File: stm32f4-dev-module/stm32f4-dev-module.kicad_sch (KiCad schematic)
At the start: 38 parts, among them J1 SW, J2 Screw_Terminal_CAN, J3 I2C1, J4 SPI1, P1 USB_C_Plug, SW1 SW_SPST, SW2 SW_SPDT, U1 STM32F405RGT6, U2 USBLC6-2SC6, U3 SN65HVD230, U4 AP2112K-3.3, U5 ICM-42670-P, Y1 25MHz

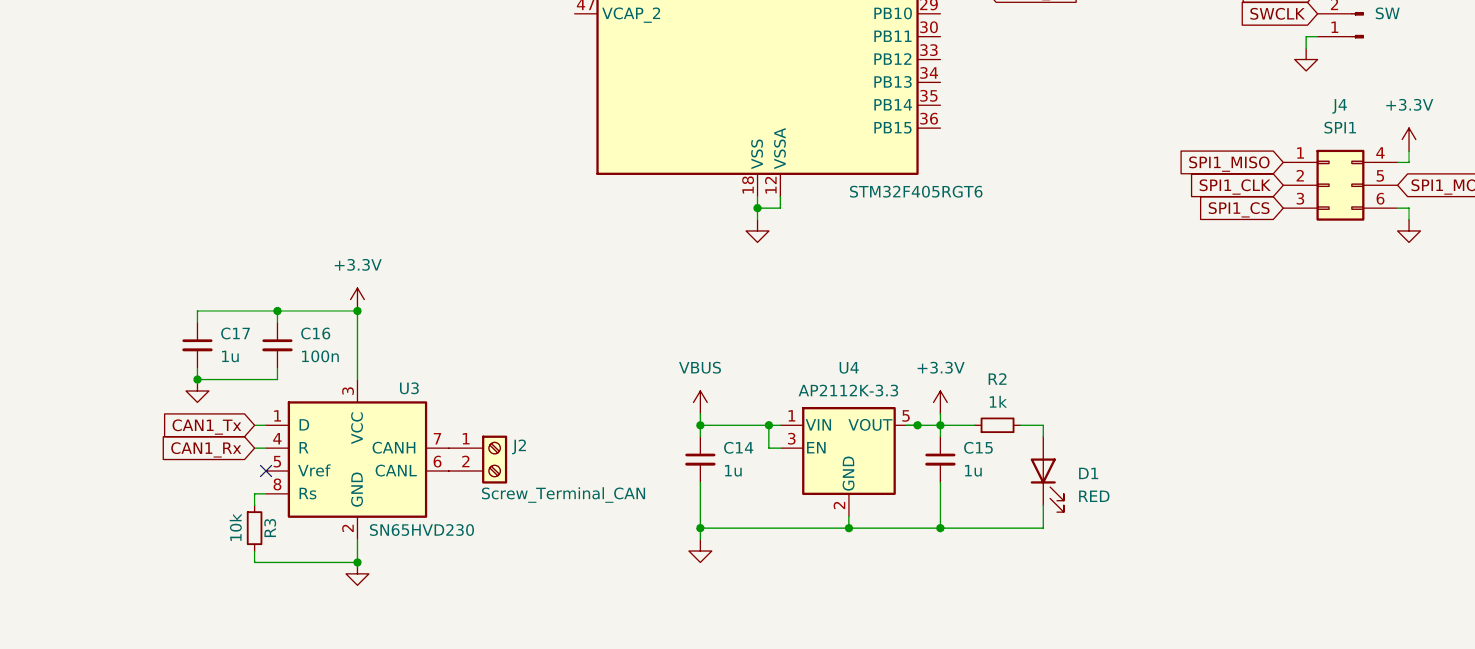
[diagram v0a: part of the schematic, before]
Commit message: commit
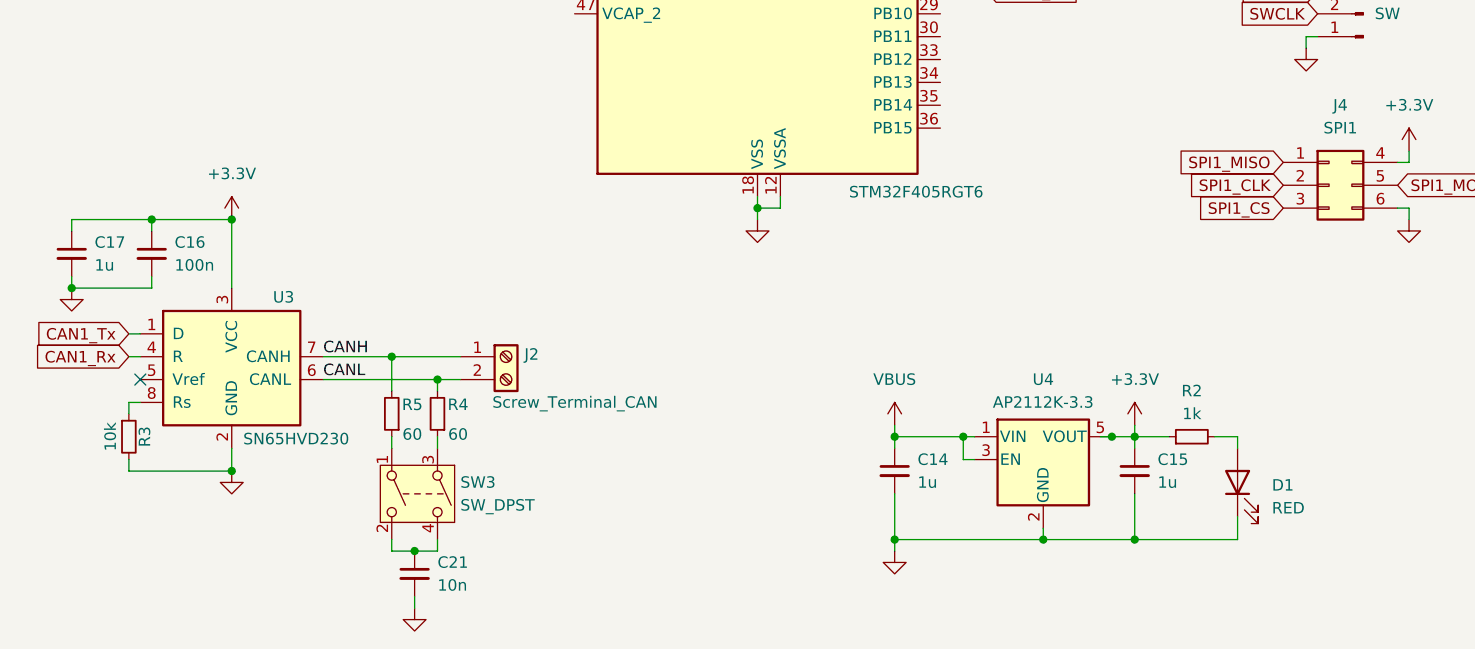
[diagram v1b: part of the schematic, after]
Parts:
- added C21: 10n, symbol Device:C_Small
- added R4, R5: 60, symbol Device:R_Small
- added SW3: SW_DPST, symbol Switch:SW_DPST
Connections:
- net GND: now also C21.2
- net CANH: now reaches J2.1 (Pin_1), U3.7 (CANH)
- net CANH: now also R5.2
- net CANL: now reaches J2.2 (Pin_2), U3.6 (CANL)
- net CANL: now also R4.2
- new net: R5.1, SW3.1
- new net: C21.1, SW3.2, SW3.4
- new net: R4.1, SW3.3
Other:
- moved on the sheet: C14, C15, C16, C17, D1, J2, R2, R3, U3, U4
